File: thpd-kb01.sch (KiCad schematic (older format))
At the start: 23 parts, among them J1 USB_C_Receptacle_USB2.0, SW1 SW_SPDT, SW2 SW_Push, U1 STM32F072C8Tx, U2 USBLC6-2SC6, U3 XC6206PxxxMR

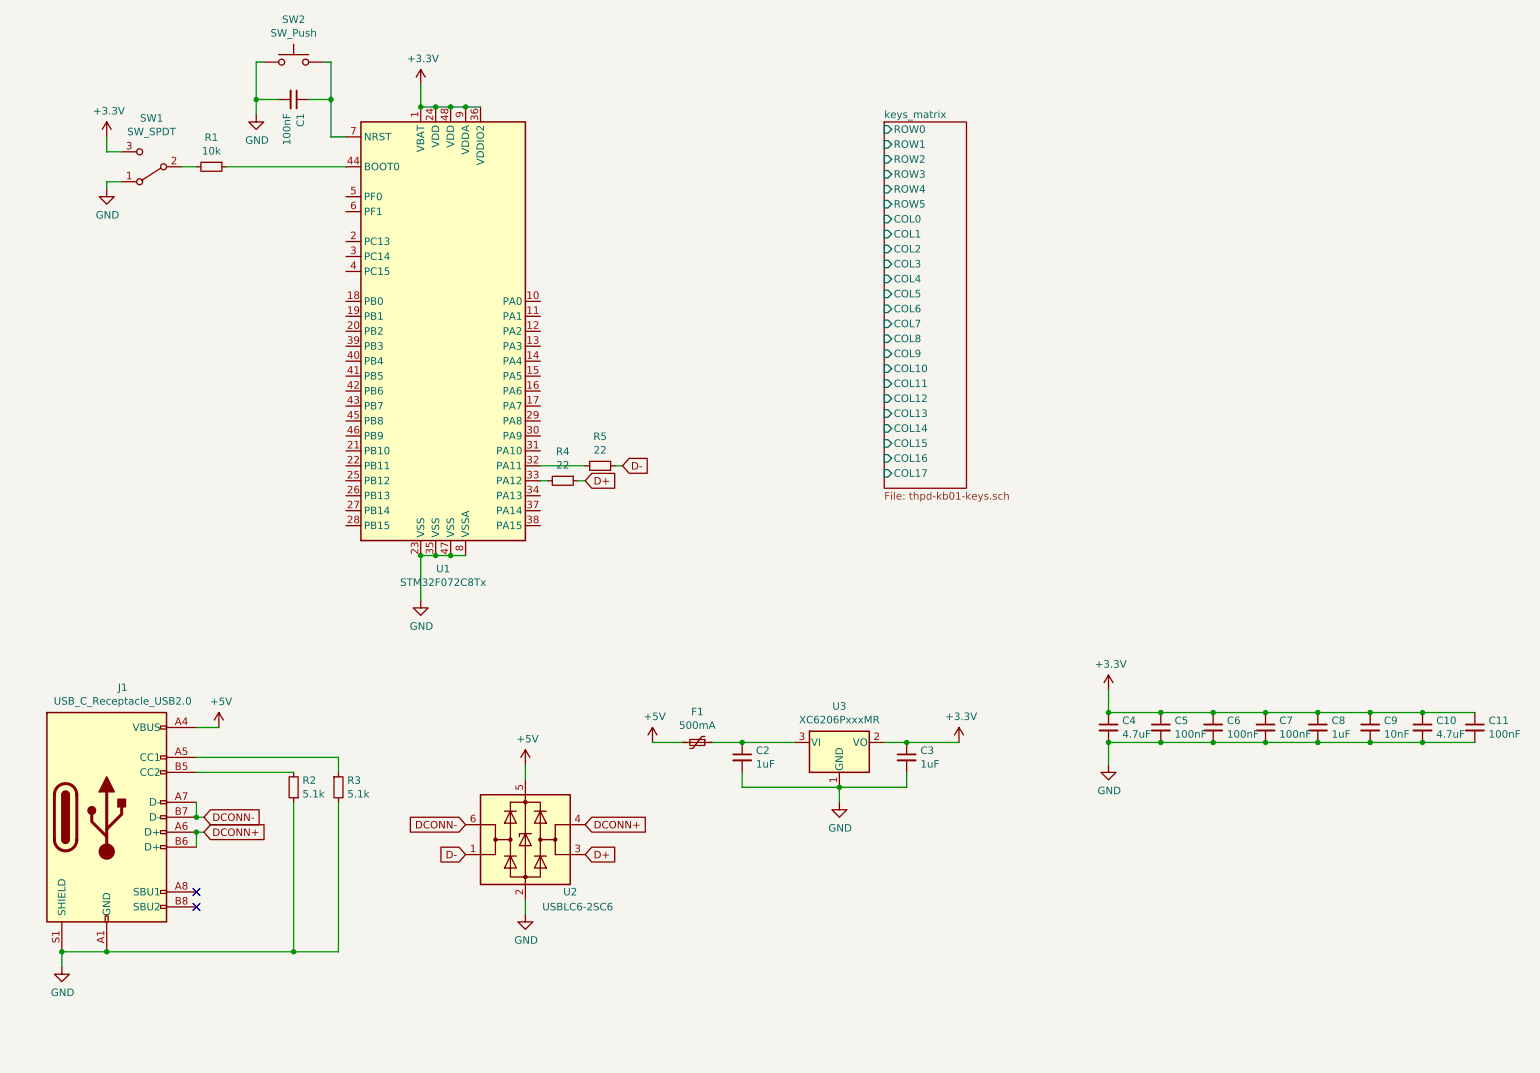
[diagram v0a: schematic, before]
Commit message: Big changes
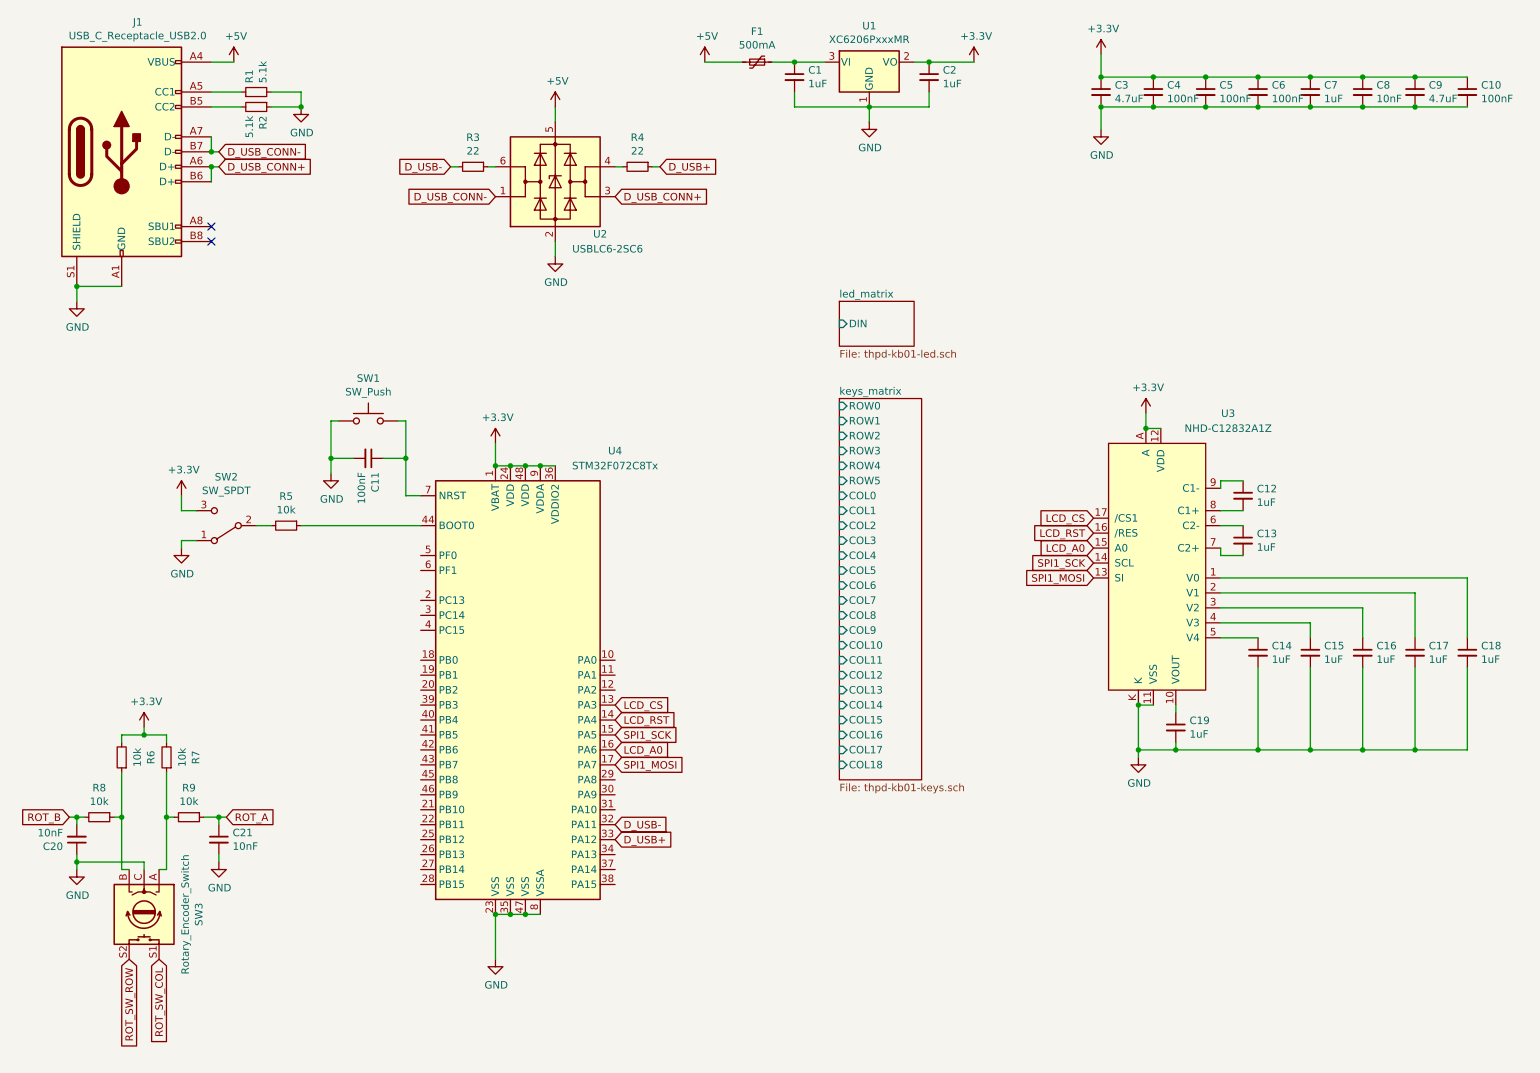
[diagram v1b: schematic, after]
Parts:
- removed R3: 5.1k, Resistor_SMD:R_0805_2012Metric, symbol Device:R_Small
- added C12, C13, C14, C15, C16, C17, C18, C19: 1uF, Capacitor_SMD:C_0402_1005Metric, symbol Device:C_Small
- added C20, C21: 10nF, Capacitor_SMD:C_0402_1005Metric, symbol Device:C_Small
- added R1: 5.1k, Resistor_SMD:R_0402_1005Metric, symbol Device:R_Small
- added R6, R7, R8, R9: 10k, Resistor_SMD:R_0603_1608Metric, symbol Device:R_Small
- added SW3: Rotary_Encoder_Switch, Rotary_Encoder:RotaryEncoder_Alps_EC11E-Switch_Vertical_H20mm, symbol Device:Rotary_Encoder_Switch
- added U3: NHD-C12832A1Z, thpd-kb01-custom:NHD-C12832A1Z, symbol thpd-kb01-custom:NHD-C12832A1Z
- C1: renamed from C2; footprint (none) -> Capacitor_SMD:C_0402_1005Metric
- C10: renamed from C11; footprint (none) -> Capacitor_SMD:C_0402_1005Metric
- C11: renamed from C1; footprint (none) -> Capacitor_SMD:C_0402_1005Metric
- C2: renamed from C3; footprint (none) -> Capacitor_SMD:C_0402_1005Metric
- C3: renamed from C4; footprint (none) -> Capacitor_SMD:C_0402_1005Metric
- C4: renamed from C5; footprint (none) -> Capacitor_SMD:C_0402_1005Metric
- C5: renamed from C6; footprint (none) -> Capacitor_SMD:C_0402_1005Metric
- C6: renamed from C7; footprint (none) -> Capacitor_SMD:C_0402_1005Metric
- C7: renamed from C8; footprint (none) -> Capacitor_SMD:C_0402_1005Metric
- C8: renamed from C9; footprint (none) -> Capacitor_SMD:C_0402_1005Metric
- C9: renamed from C10; footprint (none) -> Capacitor_SMD:C_0402_1005Metric
- R2: footprint Resistor_SMD:R_0805_2012Metric -> Resistor_SMD:R_0402_1005Metric
- R3: renamed from R5; footprint (none) -> Resistor_SMD:R_0402_1005Metric
- R4: footprint (none) -> Resistor_SMD:R_0402_1005Metric
- R5: renamed from R1; footprint (none) -> Resistor_SMD:R_0603_1608Metric
- SW1: renamed from SW2; footprint (none) -> Button_Switch_SMD:SW_Push_SPST_NO_Alps_SKRK
- SW2: renamed from SW1; footprint (none) -> thpd-kb01-custom:SW_SPDT_K3-1296S-E1
- renumbered U3 to U1, U1 to U4
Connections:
- net +3V3: now also R6.2, R7.2, U3.12 (VDD), U3.A
- net GND: now also C14.2, C15.2, C16.2, C17.2, C18.2, C19.2, C20.1, C21.2, R1.2, SW3.C, U3.11 (VSS), U3.K
- net at J1.A5 (CC1): now also R1.1
- net LCD_CS: now reaches U4.13 (PA3)
- net LCD_CS: now also U3.17 (/CS1)
- net LCD_RST: now reaches U4.14 (PA4)
- net LCD_RST: now also U3.16 (/RES)
- net SPI1_SCK: now reaches U4.15 (PA5)
- net SPI1_SCK: now also U3.14 (SCL)
- net LCD_A0: now reaches U4.16 (PA6)
- net LCD_A0: now also U3.15 (A0)
- net SPI1_MOSI: now reaches U4.17 (PA7)
- net SPI1_MOSI: now also U3.13 (SI)
- net D_USB-: now reaches R3.2, U4.32 (PA11)
- net at R4.2: now also U2.4 (I/O2); no longer U4.33 (PA12)
- net D+ renamed D_USB+
- net D_USB+: now also U4.33 (PA12); no longer U2.3 (I/O2)
- net D-: no longer names the net of R3.1
- net D-: now also U2.6 (I/O1); no longer U2.1 (I/O1)
- net DCONN+ renamed D_USB_CONN+
- net D_USB_CONN+: now also U2.3 (I/O2); no longer U2.4 (I/O2)
- net DCONN- renamed D_USB_CONN-
- net D_USB_CONN-: now also U2.1 (I/O1); no longer U2.6 (I/O1)
- new net: C18.1, U3.1 (V0)
- new net: C19.1, U3.10 (VOUT)
- new net: C17.1, U3.2 (V1)
- new net: C16.1, U3.3 (V2)
- new net: C15.1, U3.4 (V3)
- new net: C14.1, U3.5 (V4)
- new net: C13.1, U3.6 (C2-)
- new net: C13.2, U3.7 (C2+)
- new net: C12.2, U3.8 (C1+)
- new net: C12.1, U3.9 (C1-)
- new net: R7.1, R9.2, SW3.A
- new net: R6.1, R8.1, SW3.B
- new net ROT_A: C21.1, R9.1
- new net ROT_B: C20.2, R8.2
- new net ROT_SW_COL: SW3.S1
- new net ROT_SW_ROW: SW3.S2
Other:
- moved on the sheet: C1, C10, C11, C2, C3, C4, C5, C6, C7, C8, C9, F1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

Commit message: WIP
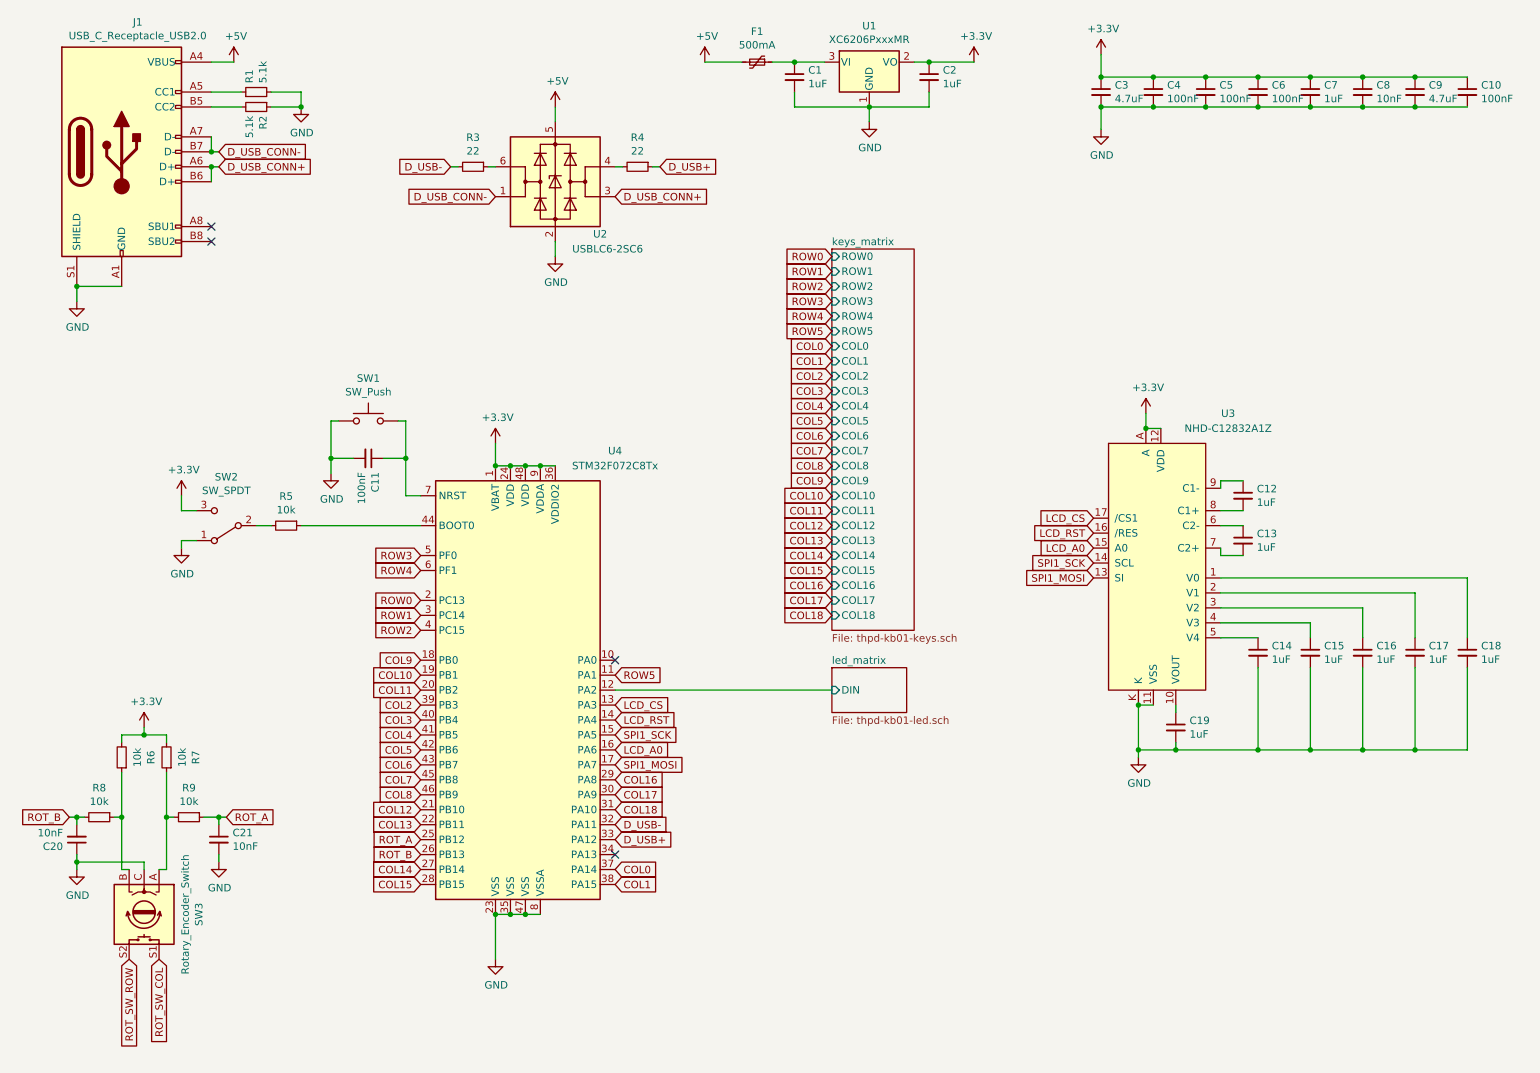
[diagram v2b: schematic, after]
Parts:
- F1: footprint Fuse:Fuse_1206_3216Metric -> Fuse:Fuse_0603_1608Metric
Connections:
- net ROT_A: now also U4.25 (PB12)
- net ROT_B: now also U4.26 (PB13)
- net led_matrix/DIN: now also U4.12 (PA2)
- net ROW5: now reaches U4.11 (PA1)
- net COL9: now reaches U4.18 (PB0)
- net COL10: now reaches U4.19 (PB1)
- net ROW0: now reaches U4.2 (PC13)
- net COL11: now reaches U4.20 (PB2)
- net COL12: now reaches U4.21 (PB10)
- net COL13: now reaches U4.22 (PB11)
- net COL14: now reaches U4.27 (PB14)
- net COL15: now reaches U4.28 (PB15)
- net COL16: now reaches U4.29 (PA8)
- net ROW1: now reaches U4.3 (PC14)
- net COL17: now reaches U4.30 (PA9)
- net COL18: now reaches U4.31 (PA10)
- net COL0: now reaches U4.37 (PA14)
- net COL1: now reaches U4.38 (PA15)
- net COL2: now reaches U4.39 (PB3)
- net ROW2: now reaches U4.4 (PC15)
- net COL3: now reaches U4.40 (PB4)
- net COL4: now reaches U4.41 (PB5)
- net COL5: now reaches U4.42 (PB6)
- net COL6: now reaches U4.43 (PB7)
- net COL7: now reaches U4.45 (PB8)
- net COL8: now reaches U4.46 (PB9)
- net ROW3: now reaches U4.5 (PF0)
- net ROW4: now reaches U4.6 (PF1)
- no-connect marks 2 -> 4
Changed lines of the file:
@@
 $EndDescr
 $Sheet
-S 6250 3400 550  2550
+S 6200 2400 550  2550
 U 618363D6
 F0 "keys_matrix" 50
 F1 "thpd-kb01-keys.sch" 50
-F2 "ROW0" I L 6250 3450 50
-F3 "ROW1" I L 6250 3550 50
-F4 "ROW2" I L 6250 3650 50
-F5 "ROW3" I L 6250 3750 50
-F6 "ROW4" I L 6250 3850 50
-F7 "ROW5" I L 6250 3950 50
-F8 "COL0" I L 6250 4050 50
-F9 "COL1" I L 6250 4150 50
-F10 "COL2" I L 6250 4250 50
-F11 "COL3" I L 6250 4350 50
-F12 "COL4" I L 6250 4450 50
-F13 "COL5" I L 6250 4550 50
-F14 "COL6" I L 6250 4650 50
-F15 "COL7" I L 6250 4750 50
-F16 "COL8" I L 6250 4850 50
-F17 "COL9" I L 6250 4950 50
-F18 "COL10" I L 6250 5050 50
-F19 "COL11" I L 6250 5150 50
-F20 "COL12" I L 6250 5250 50
-F21 "COL13" I L 6250 5350 50
-F22 "COL14" I L 6250 5450 50
-F23 "COL15" I L 6250 5550 50
-F24 "COL16" I L 6250 5650 50
-F25 "COL17" I L 6250 5750 50
-F26 "COL18" I L 6250 5850 50
+F2 "ROW0" I L 6200 2450 50
+F3 "ROW1" I L 6200 2550 50
+F4 "ROW2" I L 6200 2650 50
+F5 "ROW3" I L 6200 2750 50
+F6 "ROW4" I L 6200 2850 50
+F7 "ROW5" I L 6200 2950 50
+F8 "COL0" I L 6200 3050 50
+F9 "COL1" I L 6200 3150 50
+F10 "COL2" I L 6200 3250 50
+F11 "COL3" I L 6200 3350 50
+F12 "COL4" I L 6200 3450 50
+F13 "COL5" I L 6200 3550 50
+F14 "COL6" I L 6200 3650 50
+F15 "COL7" I L 6200 3750 50
+F16 "COL8" I L 6200 3850 50
+F17 "COL9" I L 6200 3950 50
+F18 "COL10" I L 6200 4050 50
+F19 "COL11" I L 6200 4150 50
+F20 "COL12" I L 6200 4250 50
+F21 "COL13" I L 6200 4350 50
+F22 "COL14" I L 6200 4450 50
+F23 "COL15" I L 6200 4550 50
+F24 "COL16" I L 6200 4650 50
+F25 "COL17" I L 6200 4750 50
+F26 "COL18" I L 6200 4850 50
 $EndSheet
 $Comp
@@
 F 0 "F1" V 5495 1150 50  0000 C CNN
 F 1 "500mA" V 5586 1150 50  0000 C CNN
-F 2 "Fuse:Fuse_1206_3216Metric" H 5750 950 50  0001 L CNN
+F 2 "Fuse:Fuse_0603_1608Metric" H 5750 950 50  0001 L CNN
 F 3 "~" H 5700 1150 50  0001 C CNN
 	1    5700 1150
@@
 $EndComp
 $Sheet
-S 6250 2750 500  300
+S 6200 5200 500  300
 U 625301B3
 F0 "led_matrix" 50
 F1 "thpd-kb01-led.sch" 50
-F2 "DIN" I L 6250 2900 50
+F2 "DIN" I L 6200 5350 50
 $EndSheet
 Text GLabel 1700 7150 3    50   Input ~ 0
@@
 Text GLabel 1500 7150 3    50   Input ~ 0
 ROT_SW_ROW
+Text GLabel 3450 6350 0    50   Input ~ 0
+ROT_A
+Text GLabel 3450 6450 0    50   Input ~ 0
+ROT_B
+Wire Wire Line
+	6200 5350 4750 5350
+Text GLabel 6200 2450 0    50   Input ~ 0
+ROW0
+Text GLabel 6200 2550 0    50   Input ~ 0
+ROW1
+Text GLabel 6200 2650 0    50   Input ~ 0
+ROW2
+Text GLabel 6200 2750 0    50   Input ~ 0
+ROW3
+Text GLabel 6200 2850 0    50   Input ~ 0
+ROW4
+Text GLabel 6200 2950 0    50   Input ~ 0
+ROW5
+Text GLabel 6200 3050 0    50   Input ~ 0
+COL0
+Text GLabel 6200 3150 0    50   Input ~ 0
+COL1
+Text GLabel 6200 3250 0    50   Input ~ 0
+COL2
+Text GLabel 6200 3350 0    50   Input ~ 0
+COL3
+Text GLabel 6200 3450 0    50   Input ~ 0
+COL4
+Text GLabel 6200 3550 0    50   Input ~ 0
+COL5
+Text GLabel 6200 3650 0    50   Input ~ 0
+COL6
+Text GLabel 6200 3750 0    50   Input ~ 0
+COL7
+Text GLabel 6200 3850 0    50   Input ~ 0
+COL8
+Text GLabel 6200 3950 0    50   Input ~ 0
+COL9
+Text GLabel 6200 4050 0    50   Input ~ 0
+COL10
+Text GLabel 6200 4150 0    50   Input ~ 0
+COL11
+Text GLabel 6200 4250 0    50   Input ~ 0
+COL12
+Text GLabel 6200 4350 0    50   Input ~ 0
+COL13
+Text GLabel 6200 4450 0    50   Input ~ 0
+COL14
+Text GLabel 6200 4550 0    50   Input ~ 0
+COL15
+Text GLabel 6200 4650 0    50   Input ~ 0
+COL16
+Text GLabel 6200 4750 0    50   Input ~ 0
+COL17
+Text GLabel 6200 4850 0    50   Input ~ 0
+COL18
+Text GLabel 4750 6550 2    50   Input ~ 0
+COL0
+Text GLabel 4750 6650 2    50   Input ~ 0
+COL1
+Text GLabel 3450 5450 0    50   Input ~ 0
+COL2
+Text GLabel 3450 5550 0    50   Input ~ 0
+COL3
+Text GLabel 3450 5650 0    50   Input ~ 0
+COL4
+Text GLabel 3450 5750 0    50   Input ~ 0
+COL5
+Text GLabel 3450 5850 0    50   Input ~ 0
+COL6
+Text GLabel 3450 5950 0    50   Input ~ 0
+COL7
+Text GLabel 3450 6050 0    50   Input ~ 0
+COL8
+Text GLabel 3450 5150 0    50   Input ~ 0
+COL9
+Text GLabel 3450 5250 0    50   Input ~ 0
+COL10
+Text GLabel 3450 5350 0    50   Input ~ 0
+COL11
+Text GLabel 3450 6150 0    50   Input ~ 0
+COL12
+Text GLabel 3450 6250 0    50   Input ~ 0
+COL13
+Text GLabel 3450 6550 0    50   Input ~ 0
+COL14
+Text GLabel 3450 6650 0    50   Input ~ 0
+COL15
+Text GLabel 4750 5950 2    50   Input ~ 0
+COL16
+Text GLabel 4750 6050 2    50   Input ~ 0
+COL17
+Text GLabel 4750 6150 2    50   Input ~ 0
+COL18
+Text GLabel 3450 4750 0    50   Input ~ 0
+ROW0
+Text GLabel 3450 4850 0    50   Input ~ 0
+ROW1
+Text GLabel 3450 4950 0    50   Input ~ 0
+ROW2
+Text GLabel 3450 4450 0    50   Input ~ 0
+ROW3
+Text GLabel 3450 4550 0    50   Input ~ 0
+ROW4
+Text GLabel 4750 5250 2    50   Input ~ 0
+ROW5
+NoConn ~ 4750 5150
+NoConn ~ 4750 6450
 $EndSCHEMATC
